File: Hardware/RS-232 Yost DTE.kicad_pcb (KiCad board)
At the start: 2 copper layers, 26 x 50.5 mm, 24 parts, among them J1 Conn_01x06_Female, J2 RJ45, P1 USB_C_Plug_USB2.0, U1 HIN213EIAZ, U2 FT231XS-R

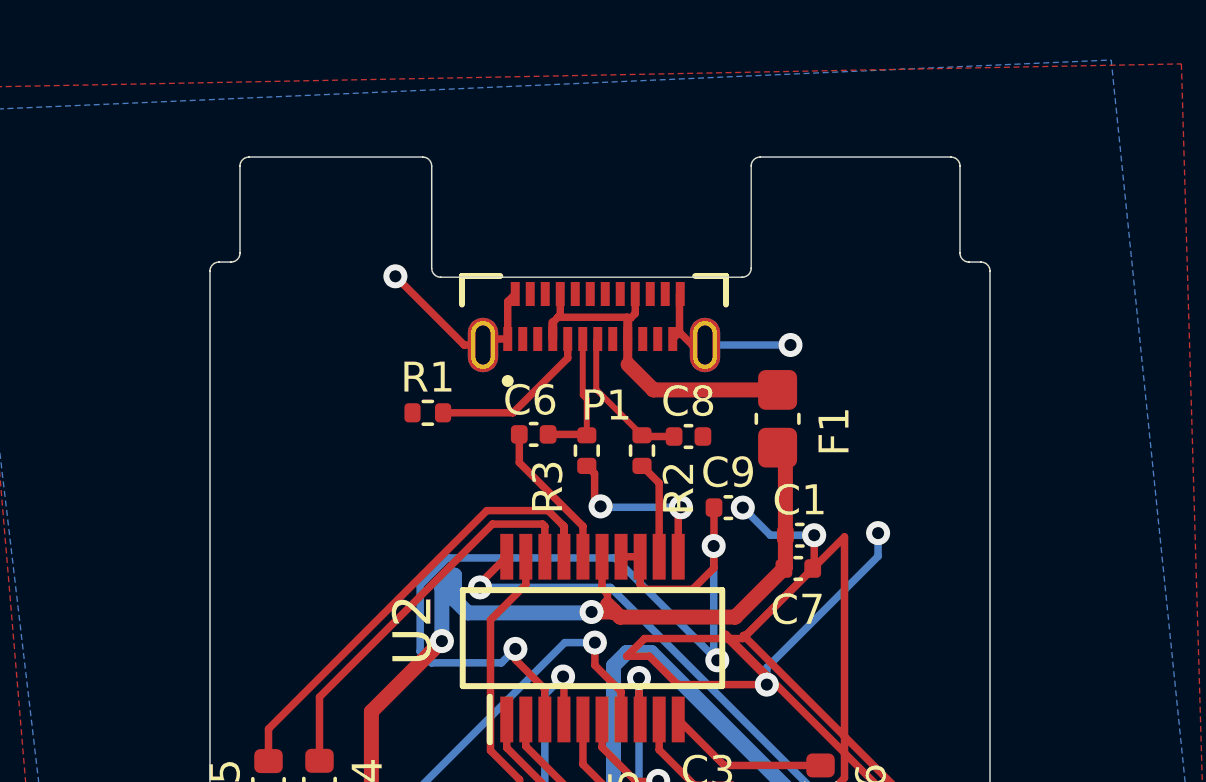
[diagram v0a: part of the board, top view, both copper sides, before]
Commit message: Updated files
Centering
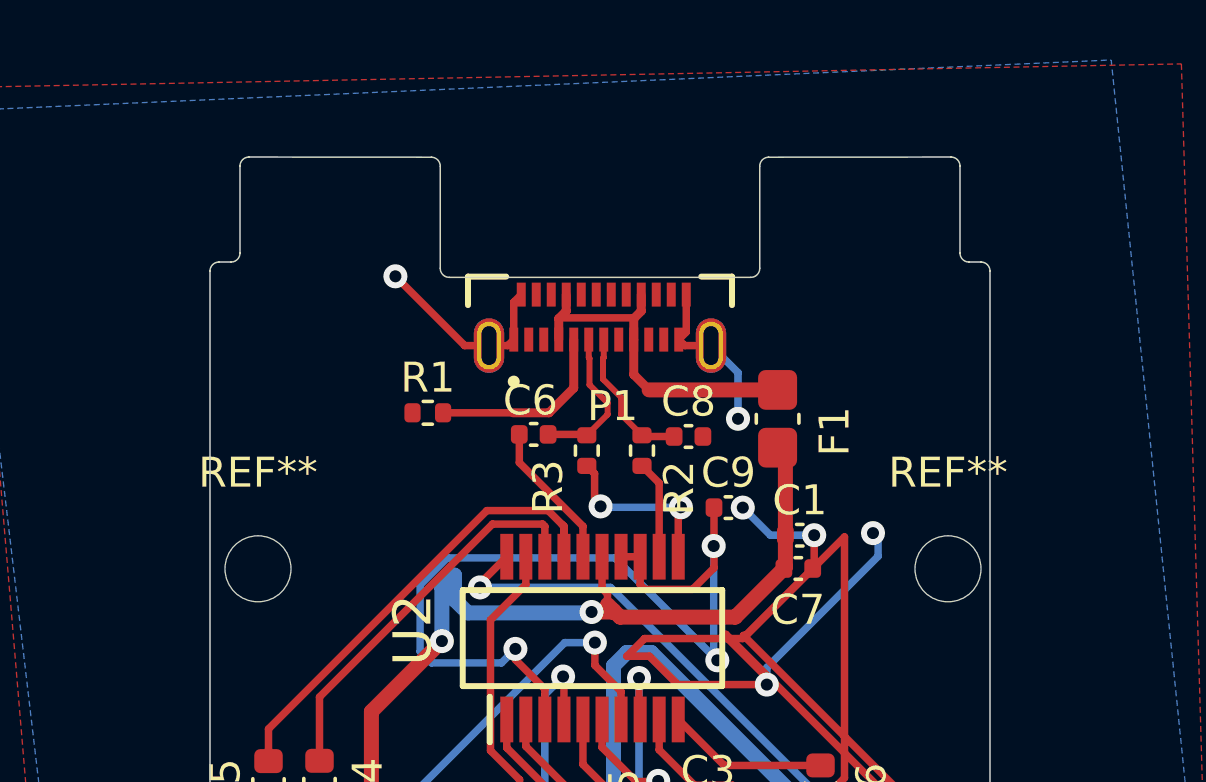
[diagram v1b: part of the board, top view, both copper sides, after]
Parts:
- added REF**: MountingHole_2.2mm_M2, MountingHole:MountingHole_2.2mm_M2, F.Cu at (140.5, 116.5)
- added REF**: MountingHole_2.2mm_M2, MountingHole:MountingHole_2.2mm_M2, F.Cu at (163.5, 116.5)
- moved P1 0.20 mm to (151.9, 108.1)
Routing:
- net Net-(P1-PadA5): track 5.55 -> 6.31 mm
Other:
- outline, holes or cut-outs redrawn
